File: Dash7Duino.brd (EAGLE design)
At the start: 100 x 80 mm, 18 parts, among them IC2 ATMEGA328", J1 POWER_JACK"

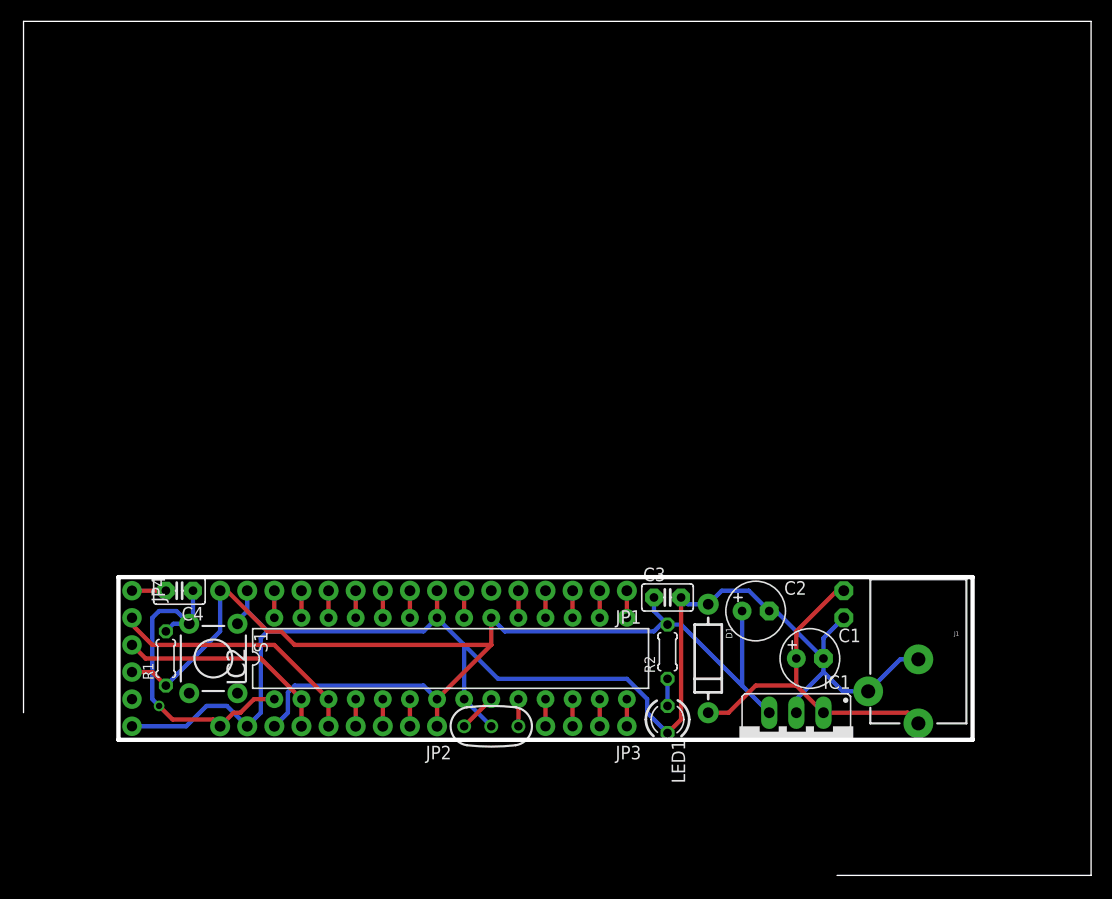
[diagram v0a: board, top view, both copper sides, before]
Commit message: almost done
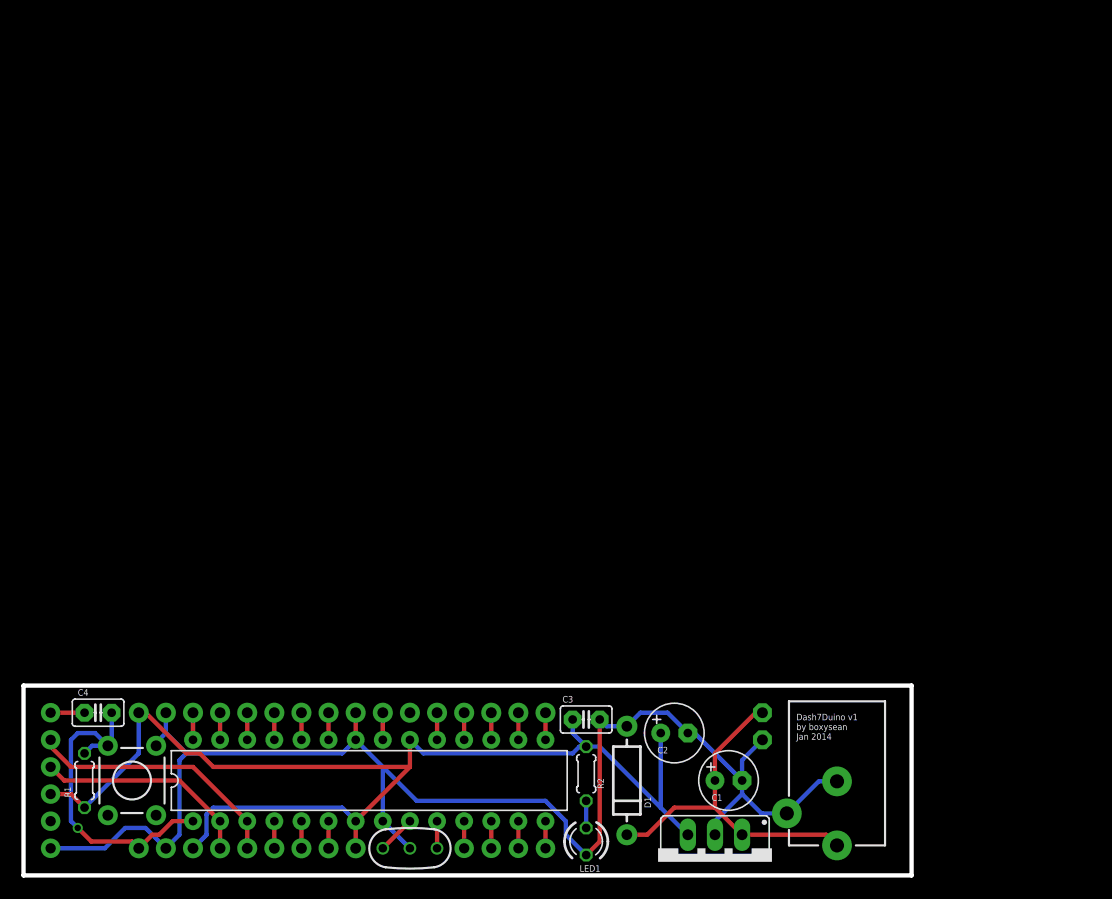
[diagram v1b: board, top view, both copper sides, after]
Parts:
- moved C3 13.7 mm to (52.7, 14.6)
- moved C4 13.7 mm to (6.99, 15.2)
- moved D1 13.7 mm to (56.5, 8.89)
- moved IC1 13.7 mm to (64.8, 1.27)
- moved IC2 13.7 mm to (32.4, 8.89)
- moved JP4 13.7 mm to (2.54, 15.2)
- moved LED1 13.7 mm to (52.7, 3.17)
- moved R2 13.7 mm to (52.7, 9.53)
- moved JP1 13.7 mm to (48.9, 15.2)
- moved JP2 13.7 mm to (31.1, 2.54)
- moved R1 13.7 mm to (5.71, 8.89)
- moved S1 13.7 mm to (10.2, 8.89)
- moved C2 13.7 mm to (61.0, 13.3)
- moved JP3 13.7 mm to (48.9, 2.54)
- moved U$2 13.7 mm to (36.2, 2.54)
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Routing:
- net +5V: vias 2 -> 0
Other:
- board size 100 x 80 mm -> 83.2 x 17.8 mm
- board text added: "/home/boxysean/Desktop/Dash7.bmp"
- board text added: "Dash7Duino v1 by boxysean Jan 2014"
